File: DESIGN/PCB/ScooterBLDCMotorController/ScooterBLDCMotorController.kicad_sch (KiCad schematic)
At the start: 30 parts, among them J1 M1 OUTPUT, J10 RC_ENABLE, J2 M1 INPUT, J3 M2 INPUT, J4 M2 OUTPUT, J5 I2C, J6 TEST SWITCH, J7 RC CH 1, J8 RC CH 2, J9 RC_PWR, U1 , U10 , U2 SN74HC14NR, U3 , U4 Teensy4.0, U5 SN74HC14NR, U6 , U7 5V_Voltage_Regulator, U8 3.3V_Voltage_Regulator, U9 

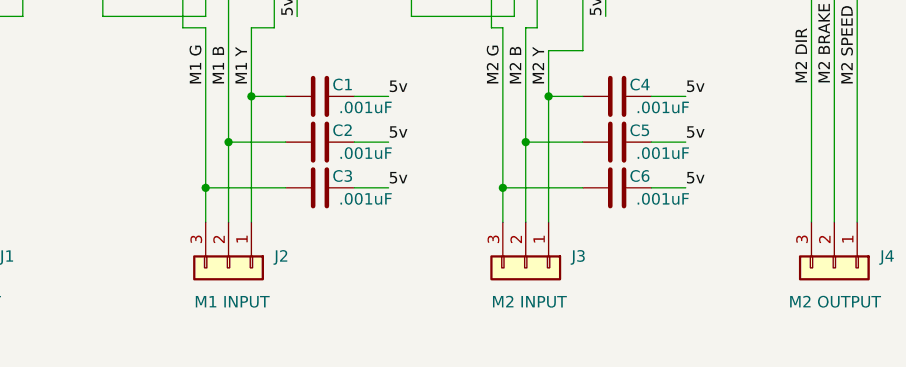
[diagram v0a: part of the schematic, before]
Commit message: Latest PCB and Rev1.0 release
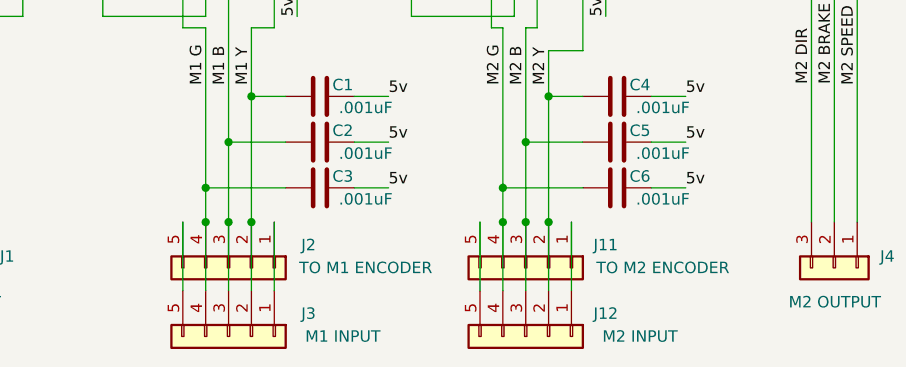
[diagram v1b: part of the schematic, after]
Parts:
- removed J2: M1 INPUT, Connector_JST:JST_XH_B3B-XH-A_1x03_P2.50mm_Vertical, symbol Connector_Generic:Conn_01x03
- removed J3: M2 INPUT, Connector_JST:JST_XH_B3B-XH-A_1x03_P2.50mm_Vertical, symbol Connector_Generic:Conn_01x03
- added J11: TO M2 ENCODER, Connector_JST:JST_XH_B5B-XH-A_1x05_P2.50mm_Vertical, symbol Connector_Generic:Conn_01x05
- added J12: M2 INPUT, Connector_JST:JST_XH_B5B-XH-A_1x05_P2.50mm_Vertical, symbol Connector_Generic:Conn_01x05
- added J2: TO M1 ENCODER, Connector_JST:JST_XH_B5B-XH-A_1x05_P2.50mm_Vertical, symbol Connector_Generic:Conn_01x05
- added J3: M1 INPUT, Connector_JST:JST_XH_B5B-XH-A_1x05_P2.50mm_Vertical, symbol Connector_Generic:Conn_01x05
- R1: footprint Resistor_THT:R_Axial_DIN0204_L3.6mm_D1.6mm_P5.08mm_Vertical -> Resistor_THT:R_Axial_DIN0204_L3.6mm_D1.6mm_P7.62mm_Horizontal
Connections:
- net M1 B: now also J2.3 (Pin_3), J3.3 (Pin_3)
- net M1 G: now also J2.4 (Pin_4), J3.4 (Pin_4)
- net M1 Y: now also J2.2 (Pin_2), J3.2 (Pin_2)
- net M2 B: now also J11.3 (Pin_3), J12.3 (Pin_3)
- net M2 G: now also J11.4 (Pin_4), J12.4 (Pin_4)
- net M2 Y: now also J11.2 (Pin_2), J12.2 (Pin_2)
- new net: J11.1 (Pin_1), J12.1 (Pin_1)
- new net: J11.5 (Pin_5), J12.5 (Pin_5)
- new net: J2.1 (Pin_1), J3.1 (Pin_1)
- new net: J2.5 (Pin_5), J3.5 (Pin_5)
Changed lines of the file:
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@@
   (junction (at 71.12 177.8) (diameter 0) (color 0 0 0 0)
   )
+  (junction (at 71.12 181.61) (diameter 0) (color 0 0 0 0)
+  )
   (junction (at 109.22 167.64) (diameter 0) (color 0 0 0 0)
   )
@@
   (junction (at 106.68 172.72) (diameter 0) (color 0 0 0 0)
   )
+  (junction (at 104.14 181.61) (diameter 0) (color 0 0 0 0)
+  )
+  (junction (at 73.66 181.61) (diameter 0) (color 0 0 0 0)
+  )
+  (junction (at 76.2 181.61) (diameter 0) (color 0 0 0 0)
+  )
   (junction (at 203.2 96.52) (diameter 0) (color 0 0 0 0)
   )
   (junction (at 104.14 177.8) (diameter 0) (color 0 0 0 0)
   )
+  (junction (at 106.68 181.61) (diameter 0) (color 0 0 0 0)
+  )
+  (junction (at 109.22 181.61) (diameter 0) (color 0 0 0 0)
+  )
   (wire (pts (xy 85.09 140.97) (xy 81.28 140.97))
     (stroke (width 0) (type default) (color 0 0 0 0))
@@
     (stroke (width 0) (type default) (color 0 0 0 0))
   )
+  (wire (pts (xy 109.22 181.61) (xy 109.22 189.23))
+    (stroke (width 0) (type default) (color 0 0 0 0))
+  )
   (wire (pts (xy 133.35 115.57) (xy 133.35 99.06))
     (stroke (width 0) (type default) (color 0 0 0 0))
@@
     (stroke (width 0) (type default) (color 0 0 0 0))
   )
+  (wire (pts (xy 78.74 181.61) (xy 78.74 189.23))
+    (stroke (width 0) (type default) (color 0 0 0 0))
+  )
   (wire (pts (xy 177.8 26.67) (xy 177.8 15.24))
     (stroke (width 0) (type default) (color 0 0 0 0))
@@
     (stroke (width 0) (type default) (color 0 0 0 0))
   )
+  (wire (pts (xy 71.12 181.61) (xy 71.12 189.23))
+    (stroke (width 0) (type default) (color 0 0 0 0))
+  )
   (wire (pts (xy 45.72 133.35) (xy 45.72 130.81))
     (stroke (width 0) (type default) (color 0 0 0 0))
@@
     (stroke (width 0) (type default) (color 0 0 0 0))
   )
+  (wire (pts (xy 101.6 181.61) (xy 101.6 189.23))
+    (stroke (width 0) (type default) (color 0 0 0 0))
+  )
   (wire (pts (xy 205.74 59.69) (xy 190.5 59.69))
     (stroke (width 0) (type default) (color 0 0 0 0))
@@
     (stroke (width 0) (type default) (color 0 0 0 0))
   )
+  (wire (pts (xy 111.76 181.61) (xy 111.76 189.23))
+    (stroke (width 0) (type default) (color 0 0 0 0))
+  )
   (wire (pts (xy 69.85 83.82) (xy 69.85 88.9))
     (stroke (width 0) (type default) (color 0 0 0 0))
@@
     (stroke (width 0) (type default) (color 0 0 0 0))
   )
+  (wire (pts (xy 73.66 181.61) (xy 73.66 189.23))
+    (stroke (width 0) (type default) (color 0 0 0 0))
+  )
   (wire (pts (xy 113.03 154.94) (xy 113.03 162.56))
     (stroke (width 0) (type default) (color 0 0 0 0))
@@
     (stroke (width 0) (type default) (color 0 0 0 0))
   )
+  (wire (pts (xy 104.14 181.61) (xy 104.14 189.23))
+    (stroke (width 0) (type default) (color 0 0 0 0))
+  )
   (wire (pts (xy 90.17 130.81) (xy 90.17 133.35))
     (stroke (width 0) (type default) (color 0 0 0 0))
@@
     (stroke (width 0) (type default) (color 0 0 0 0))
   )
+  (wire (pts (xy 68.58 181.61) (xy 68.58 189.23))
+    (stroke (width 0) (type default) (color 0 0 0 0))
+  )
   (wire (pts (xy 97.79 106.68) (xy 85.09 106.68))
     (stroke (width 0) (type default) (color 0 0 0 0))
@@
     (stroke (width 0) (type default) (color 0 0 0 0))
   )
+  (wire (pts (xy 106.68 181.61) (xy 106.68 189.23))
+    (stroke (width 0) (type default) (color 0 0 0 0))
+  )
   (wire (pts (xy 248.92 54.61) (xy 240.03 54.61))
     (stroke (width 0) (type default) (color 0 0 0 0))
@@
   )
   (wire (pts (xy 245.11 44.45) (xy 252.73 44.45))
+    (stroke (width 0) (type default) (color 0 0 0 0))
+  )
+  (wire (pts (xy 76.2 181.61) (xy 76.2 189.23))
     (stroke (width 0) (type default) (color 0 0 0 0))
   )
@@
     (pin "9")
   )
+  (symbol (lib_id "Connector_Generic:Conn_01x05") (at 106.68 194.31 270) (unit 1)
+    (in_bom yes) (on_board yes)
+    (property "Reference" "J12" (id 0) (at 115.57 191.77 90))
+    (property "Value" "M2 INPUT" (id 1) (at 119.38 194.31 90))
+    (property "Footprint" "Connector_JST:JST_XH_B5B-XH-A_1x05_P2.50mm_Vertical" (id 2) (at 106.68 194.31 0)
+      (effects (font (size 1.27 1.27)) hide)
+    )
+    (property "Datasheet" "~" (id 3) (at 106.68 194.31 0)
+      (effects (font (size 1.27 1.27)) hide)
+    )
+    (pin "1")
+    (pin "2")
+    (pin "3")
+    (pin "4")
+    (pin "5")
+  )
+  (symbol (lib_id "Connector_Generic:Conn_01x05") (at 73.66 186.69 270) (unit 1)
+    (in_bom yes) (on_board yes)
+    (property "Reference" "J2" (id 0) (at 82.55 184.15 90))
+    (property "Value" "TO M1 ENCODER" (id 1) (at 88.9 186.69 90))
+    (property "Footprint" "Connector_JST:JST_XH_B5B-XH-A_1x05_P2.50mm_Vertical" (id 2) (at 73.66 186.69 0)
+      (effects (font (size 1.27 1.27)) hide)
+    )
+    (property "Datasheet" "~" (id 3) (at 73.66 186.69 0)
+      (effects (font (size 1.27 1.27)) hide)
+    )
+    (pin "1")
+    (pin "2")
+    (pin "3")
+    (pin "4")
+    (pin "5")
+  )
   (symbol (lib_id "Custom:Level_Shifter") (at 171.45 34.29 90) (unit 1)
     (in_bom yes) (on_board yes) (fields_autoplaced)
@@
     (property "Reference" "R1" (id 0) (at 193.04 99.06 90))
     (property "Value" "R" (id 1) (at 193.04 96.52 90))
-    (property "Footprint" "Resistor_THT:R_Axial_DIN0204_L3.6mm_D1.6mm_P5.08mm_Vertical" (id 2) (at 193.04 98.298 90)
+    (property "Footprint" "Resistor_THT:R_Axial_DIN0204_L3.6mm_D1.6mm_P7.62mm_Horizontal" (id 2) (at 193.04 98.298 90)
       (effects (font (size 1.27 1.27)) hide)
     )
@@
     (pin "4")
   )
-  (symbol (lib_id "Connector_Generic:Conn_01x03") (at 106.68 186.69 270) (unit 1)
-    (in_bom yes) (on_board yes)
-    (property "Reference" "J3" (id 0) (at 111.76 185.4199 90)
-      (effects (font (size 1.27 1.27)) (justify left))
-    )
-    (property "Value" "M2 INPUT" (id 1) (at 102.87 190.5 90)
-      (effects (font (size 1.27 1.27)) (justify left))
-    )
-    (property "Footprint" "Connector_JST:JST_XH_B3B-XH-A_1x03_P2.50mm_Vertical" (id 2) (at 106.68 186.69 0)
+  (symbol (lib_id "Connector_Generic:Conn_01x05") (at 106.68 186.69 270) (unit 1)
+    (in_bom yes) (on_board yes)
+    (property "Reference" "J11" (id 0) (at 115.57 184.15 90))
+    (property "Value" "TO M2 ENCODER" (id 1) (at 121.92 186.69 90))
+    (property "Footprint" "Connector_JST:JST_XH_B5B-XH-A_1x05_P2.50mm_Vertical" (id 2) (at 106.68 186.69 0)
       (effects (font (size 1.27 1.27)) hide)
     )
@@
     (pin "2")
     (pin "3")
+    (pin "4")
+    (pin "5")
   )
   (symbol (lib_id "Custom:SN74HC14NR") (at 107.95 151.13 270) (unit 1)
@@
     (pin "9")
   )
+  (symbol (lib_id "Connector_Generic:Conn_01x05") (at 73.66 194.31 270) (unit 1)
+    (in_bom yes) (on_board yes)
+    (property "Reference" "J3" (id 0) (at 82.55 191.77 90))
+    (property "Value" "M1 INPUT" (id 1) (at 86.36 194.31 90))
+    (property "Footprint" "Connector_JST:JST_XH_B5B-XH-A_1x05_P2.50mm_Vertical" (id 2) (at 73.66 194.31 0)
+      (effects (font (size 1.27 1.27)) hide)
+    )
+    (property "Datasheet" "~" (id 3) (at 73.66 194.31 0)
+      (effects (font (size 1.27 1.27)) hide)
+    )
+    (pin "1")
+    (pin "2")
+    (pin "3")
+    (pin "4")
+    (pin "5")
+  )
   (symbol (lib_id "Device:C") (at 116.84 172.72 270) (unit 1)
     (in_bom yes) (on_board yes)
@@
     (pin "1")
     (pin "2")
-  )
-  (symbol (lib_id "Connector_Generic:Conn_01x03") (at 73.66 186.69 270) (unit 1)
-    (in_bom yes) (on_board yes)
-    (property "Reference" "J2" (id 0) (at 78.74 185.4199 90)
-      (effects (font (size 1.27 1.27)) (justify left))
-    )
-    (property "Value" "M1 INPUT" (id 1) (at 69.85 190.5 90)
-      (effects (font (size 1.27 1.27)) (justify left))
-    )
-    (property "Footprint" "Connector_JST:JST_XH_B3B-XH-A_1x03_P2.50mm_Vertical" (id 2) (at 73.66 186.69 0)
-      (effects (font (size 1.27 1.27)) hide)
-    )
-    (property "Datasheet" "~" (id 3) (at 73.66 186.69 0)
-      (effects (font (size 1.27 1.27)) hide)
-    )
-    (pin "1")
-    (pin "2")
-    (pin "3")
   )
   (symbol (lib_id "Custom:3.3V_Voltage_Regulator") (at 252.73 40.64 90) (unit 1)
@@
       (reference "J1") (unit 1) (value "M1 OUTPUT") (footprint "Connector_JST:JST_XH_B3B-XH-A_1x03_P2.50mm_Vertical")
     )
-    (path "/c803ae01-d083-4855-8801-39dea92f7d1b"
-      (reference "J2") (unit 1) (value "M1 INPUT") (footprint "Connector_JST:JST_XH_B3B-XH-A_1x03_P2.50mm_Vertical")
-    )
-    (path "/9925a326-63ef-4346-b01c-a42c2e49fa06"
-      (reference "J3") (unit 1) (value "M2 INPUT") (footprint "Connector_JST:JST_XH_B3B-XH-A_1x03_P2.50mm_Vertical")
+    (path "/6c578b81-c5ac-40f2-828f-f316ca08e2c9"
+      (reference "J2") (unit 1) (value "TO M1 ENCODER") (footprint "Connector_JST:JST_XH_B5B-XH-A_1x05_P2.50mm_Vertical")
+    )
+    (path "/a535aaee-d403-444b-bf48-91bd8f6bbbbb"
+      (reference "J3") (unit 1) (value "M1 INPUT") (footprint "Connector_JST:JST_XH_B5B-XH-A_1x05_P2.50mm_Vertical")
     )
     (path "/18022ffe-56bf-49ac-890a-29ec31eec758"
@@
       (reference "J10") (unit 1) (value "RC_ENABLE") (footprint "Connector_PinHeader_2.54mm:PinHeader_1x02_P2.54mm_Vertical")
     )
+    (path "/9c217da1-3f00-4b6e-8b3e-d4724992586b"
+      (reference "J11") (unit 1) (value "TO M2 ENCODER") (footprint "Connector_JST:JST_XH_B5B-XH-A_1x05_P2.50mm_Vertical")
+    )
+    (path "/4811cedc-e653-4dd3-ab03-bd6ac45aea2a"
+      (reference "J12") (unit 1) (value "M2 INPUT") (footprint "Connector_JST:JST_XH_B5B-XH-A_1x05_P2.50mm_Vertical")
+    )
     (path "/121b8a59-e57c-4cdd-877c-c2b279b4ad3b"
       (reference "POWER1") (unit 1) (value "5v") (footprint "Connector_JST:JST_XH_B2B-XH-A_1x02_P2.50mm_Vertical")
     )
     (path "/8811b52e-d3c2-4783-979a-166200d19a26"
-      (reference "R1") (unit 1) (value "R") (footprint "Resistor_THT:R_Axial_DIN0204_L3.6mm_D1.6mm_P5.08mm_Vertical")
+      (reference "R1") (unit 1) (value "R") (footprint "Resistor_THT:R_Axial_DIN0204_L3.6mm_D1.6mm_P7.62mm_Horizontal")
     )
     (path "/a906d8c4-7ffd-463c-a1b9-091846f7101c"
